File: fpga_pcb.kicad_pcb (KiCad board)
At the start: 4 copper layers, 100 x 65 mm, 230 parts, among them J1 USB_C_Receptacle_USB2.0_16P, J10 Conn_02x08_Odd_Even, J11 Conn_02x08_Odd_Even, J12 5VIN, J13 Conn_01x10, J14 RJ45_Halo_HFJ11-x2450E-LxxRL, J2 Conn_01x06, J3 Conn_01x06, J4 Conn_01x06, J5 Conn_01x06, J6 Conn_01x06, J7 Conn_01x06, J8 Conn_01x06, J9 Conn_01x06, SW1 SW_Push, SW2 SW_Push, U10 LAN8720A, U11 SN74LV244AQDGSRQ1, U2 23AA02M-IST, U3 TPS62A02APDDC, U4 TLV75733PDBV, U5 TPS2116DRL, U6 93AAxxBT-xOT, U7 USBLC6-2SC6, U8 FT4232H, U9 ADC1283, Y1 ECS-2520MV-500-xx, Y2 Crystal_GND24

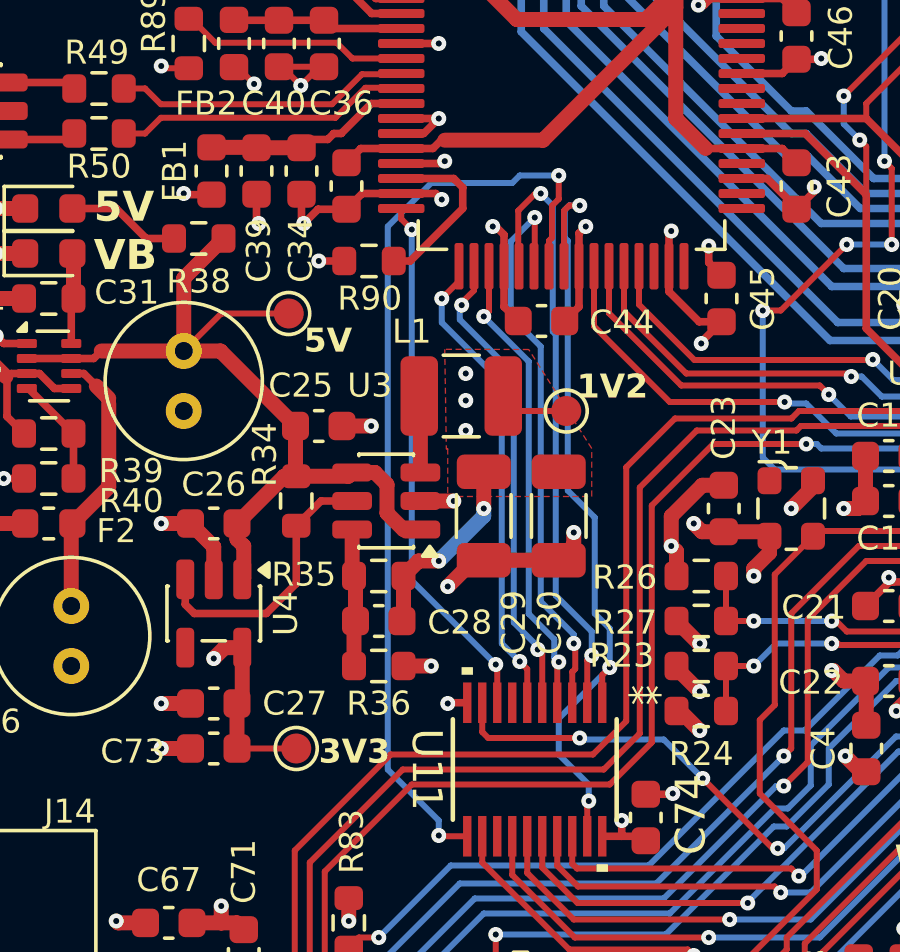
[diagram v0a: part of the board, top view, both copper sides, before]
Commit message: Finalized
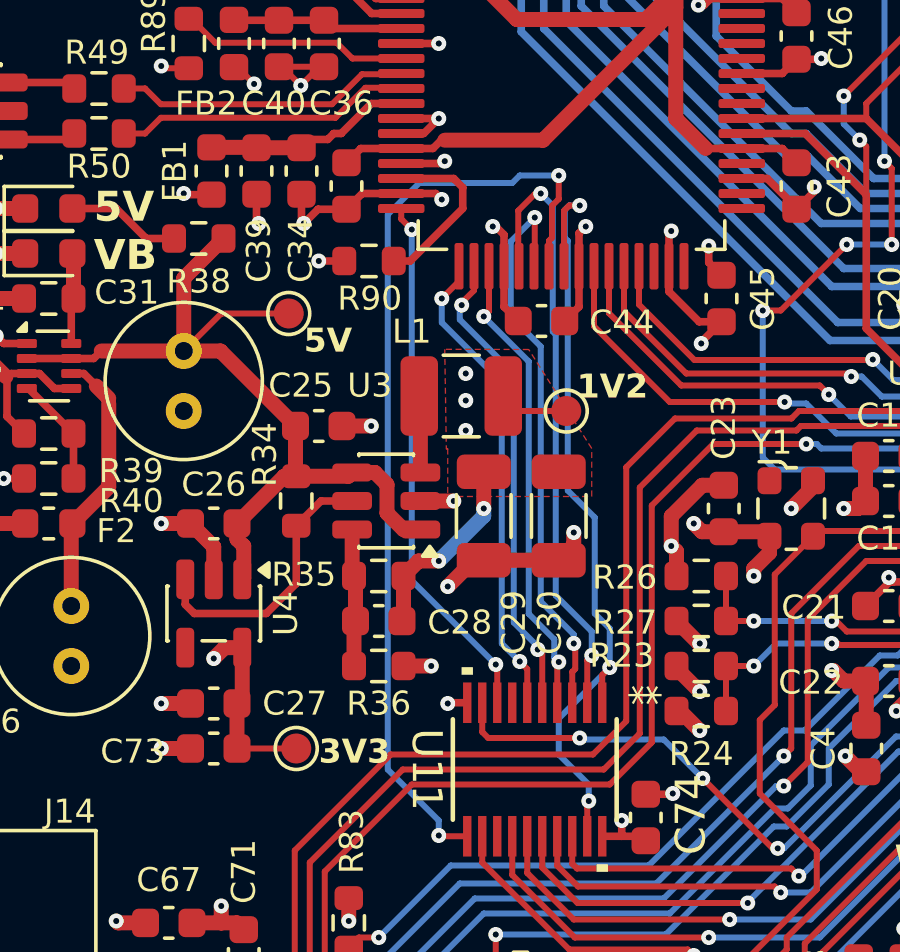
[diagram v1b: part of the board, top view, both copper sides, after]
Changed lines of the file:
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@@
 	)
 	(segment
-		(start 27.3 181.7)
-		(end 27.3 163.6)
+		(start 31.45 162.15)
+		(end 31.7 161.9)
 		(width 0.2)
 		(layer "B.Cu")
@@
 	)
 	(segment
-		(start 28.75 162.15)
-		(end 31.45 162.15)
-		(width 0.2)
-		(layer "B.Cu")
-		(net "/USB/FT_HOLD")
-	)
-	(segment
-		(start 27.3 163.6)
-		(end 28.75 162.15)
+		(start 27.3 163.2)
+		(end 28.35 162.15)
 		(width 0.2)
 		(layer "B.Cu")
@@
 	)
 	(segment
-		(start 29 183.4)
-		(end 27.3 181.7)
+		(start 28.35 162.15)
+		(end 31.45 162.15)
 		(width 0.2)
 		(layer "B.Cu")
@@
 	)
 	(segment
-		(start 31.45 162.15)
-		(end 31.7 161.9)
+		(start 27.3 181.7)
+		(end 27.3 163.2)
 		(width 0.2)
 		(layer "B.Cu")
+		(net "/USB/FT_HOLD")
+	)
+	(segment
+		(start 29 183.4)
+		(end 27.3 181.7)
+		(width 0.2)
+		(layer "B.Cu")
